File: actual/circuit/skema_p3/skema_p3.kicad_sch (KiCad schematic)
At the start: 0 parts

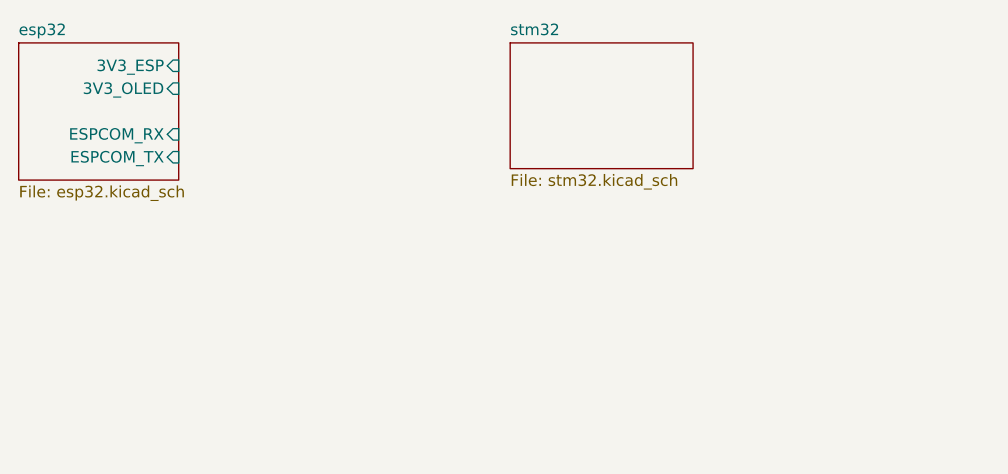
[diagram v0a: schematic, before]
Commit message: P3 in KiCAD
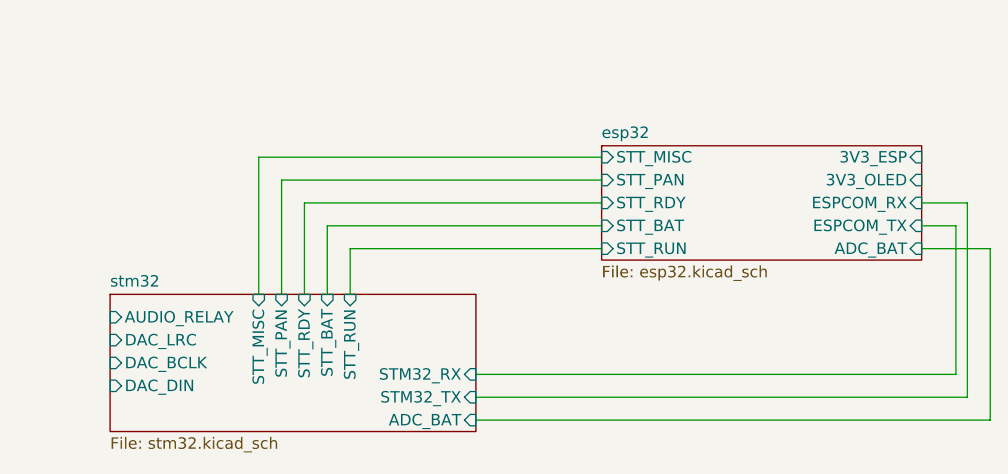
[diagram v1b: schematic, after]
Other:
- sheet esp32 ports: added ADC_BAT, STT_BAT, STT_MISC, STT_PAN, STT_RDY, STT_RUN; removed none
- sheet stm32 ports: added ADC_BAT, AUDIO_RELAY, DAC_BCLK, DAC_DIN, DAC_LRC, STM32_RX, STM32_TX, STT_BAT, STT_MISC, STT_PAN, STT_RDY, STT_RUN; removed none
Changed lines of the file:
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@@
 (kicad_sch (version 20211123) (generator eeschema)
-  (paper "User" 150.012 99.9998)
+  (paper "User" 150.012 150.012)
   (title_block
     (title "Audiometri Base Schematic")
@@
     (rev "P3 v2")
   )
-  (sheet (at 16.51 16.51) (size 17.78 15.24) (fields_autoplaced)
+  (wire (pts (xy 67.31 58.42) (xy 124.46 58.42))
+    (stroke (width 0) (type default) (color 0 0 0 0))
+  )
+  (wire (pts (xy 48.26 34.29) (xy 81.28 34.29))
+    (stroke (width 0) (type default) (color 0 0 0 0))
+  )
+  (wire (pts (xy 67.31 55.88) (xy 121.92 55.88))
+    (stroke (width 0) (type default) (color 0 0 0 0))
+  )
+  (wire (pts (xy 120.65 53.34) (xy 120.65 36.83))
+    (stroke (width 0) (type default) (color 0 0 0 0))
+  )
+  (wire (pts (xy 50.8 44.45) (xy 50.8 36.83))
+    (stroke (width 0) (type default) (color 0 0 0 0))
+  )
+  (wire (pts (xy 53.34 39.37) (xy 81.28 39.37))
+    (stroke (width 0) (type default) (color 0 0 0 0))
+  )
+  (wire (pts (xy 67.31 53.34) (xy 120.65 53.34))
+    (stroke (width 0) (type default) (color 0 0 0 0))
+  )
+  (wire (pts (xy 45.72 44.45) (xy 45.72 31.75))
+    (stroke (width 0) (type default) (color 0 0 0 0))
+  )
+  (wire (pts (xy 116.84 36.83) (xy 120.65 36.83))
+    (stroke (width 0) (type default) (color 0 0 0 0))
+  )
+  (wire (pts (xy 124.46 58.42) (xy 124.46 39.37))
+    (stroke (width 0) (type default) (color 0 0 0 0))
+  )
+  (wire (pts (xy 43.18 29.21) (xy 81.28 29.21))
+    (stroke (width 0) (type default) (color 0 0 0 0))
+  )
+  (wire (pts (xy 50.8 36.83) (xy 81.28 36.83))
+    (stroke (width 0) (type default) (color 0 0 0 0))
+  )
+  (wire (pts (xy 48.26 44.45) (xy 48.26 34.29))
+    (stroke (width 0) (type default) (color 0 0 0 0))
+  )
+  (wire (pts (xy 124.46 39.37) (xy 116.84 39.37))
+    (stroke (width 0) (type default) (color 0 0 0 0))
+  )
+  (wire (pts (xy 43.18 44.45) (xy 43.18 29.21))
+    (stroke (width 0) (type default) (color 0 0 0 0))
+  )
+  (wire (pts (xy 53.34 44.45) (xy 53.34 39.37))
+    (stroke (width 0) (type default) (color 0 0 0 0))
+  )
+  (wire (pts (xy 45.72 31.75) (xy 81.28 31.75))
+    (stroke (width 0) (type default) (color 0 0 0 0))
+  )
+  (wire (pts (xy 121.92 55.88) (xy 121.92 34.29))
+    (stroke (width 0) (type default) (color 0 0 0 0))
+  )
+  (wire (pts (xy 121.92 34.29) (xy 116.84 34.29))
+    (stroke (width 0) (type default) (color 0 0 0 0))
+  )
+  (sheet (at 81.28 27.94) (size 35.56 12.7) (fields_autoplaced)
     (stroke (width 0.1524) (type solid) (color 0 0 0 0))
     (fill (color 0 0 0 0.0000))
-    (property "Sheet name" "esp32" (id 0) (at 16.51 15.7984 0)
+    (property "Sheet name" "esp32" (id 0) (at 81.28 27.2284 0)
       (effects (font (size 1.27 1.27)) (justify left bottom))
     )
-    (property "Sheet file" "esp32.kicad_sch" (id 1) (at 16.51 32.3346 0)
+    (property "Sheet file" "esp32.kicad_sch" (id 1) (at 81.28 41.2246 0)
       (effects (font (size 1.27 1.27)) (justify left top))
     )
-    (pin "3V3_ESP" input (at 34.29 19.05 0)
-      (effects (font (size 1.27 1.27)) (justify right))
-    )
-    (pin "ESPCOM_RX" input (at 34.29 26.67 0)
-      (effects (font (size 1.27 1.27)) (justify right))
-    )
-    (pin "ESPCOM_TX" input (at 34.29 29.21 0)
-      (effects (font (size 1.27 1.27)) (justify right))
-    )
-    (pin "3V3_OLED" input (at 34.29 21.59 0)
-      (effects (font (size 1.27 1.27)) (justify right))
-    )
-  )
-  (sheet (at 71.12 16.51) (size 20.32 13.97) (fields_autoplaced)
+    (pin "3V3_ESP" input (at 116.84 29.21 0)
+      (effects (font (size 1.27 1.27)) (justify right))
+    )
+    (pin "ESPCOM_RX" input (at 116.84 34.29 0)
+      (effects (font (size 1.27 1.27)) (justify right))
+    )
+    (pin "ESPCOM_TX" input (at 116.84 36.83 0)
+      (effects (font (size 1.27 1.27)) (justify right))
+    )
+    (pin "3V3_OLED" input (at 116.84 31.75 0)
+      (effects (font (size 1.27 1.27)) (justify right))
+    )
+    (pin "STT_MISC" input (at 81.28 29.21 180)
+      (effects (font (size 1.27 1.27)) (justify left))
+    )
+    (pin "STT_PAN" input (at 81.28 31.75 180)
+      (effects (font (size 1.27 1.27)) (justify left))
+    )
+    (pin "STT_RDY" input (at 81.28 34.29 180)
+      (effects (font (size 1.27 1.27)) (justify left))
+    )
+    (pin "STT_BAT" input (at 81.28 36.83 180)
+      (effects (font (size 1.27 1.27)) (justify left))
+    )
+    (pin "STT_RUN" input (at 81.28 39.37 180)
+      (effects (font (size 1.27 1.27)) (justify left))
+    )
+    (pin "ADC_BAT" input (at 116.84 39.37 0)
+      (effects (font (size 1.27 1.27)) (justify right))
+    )
+  )
+  (sheet (at 26.67 44.45) (size 40.64 15.24) (fields_autoplaced)
     (stroke (width 0.1524) (type solid) (color 0 0 0 0))
     (fill (color 0 0 0 0.0000))
-    (property "Sheet name" "stm32" (id 0) (at 71.12 15.7984 0)
+    (property "Sheet name" "stm32" (id 0) (at 26.67 43.7384 0)
       (effects (font (size 1.27 1.27)) (justify left bottom))
     )
-    (property "Sheet file" "stm32.kicad_sch" (id 1) (at 71.12 31.0646 0)
+    (property "Sheet file" "stm32.kicad_sch" (id 1) (at 26.67 60.2746 0)
       (effects (font (size 1.27 1.27)) (justify left top))
+    )
+    (pin "STT_MISC" input (at 43.18 44.45 90)
+      (effects (font (size 1.27 1.27)) (justify right))
+    )
+    (pin "STM32_TX" input (at 67.31 55.88 0)
+      (effects (font (size 1.27 1.27)) (justify right))
+    )
+    (pin "STM32_RX" input (at 67.31 53.34 0)
+      (effects (font (size 1.27 1.27)) (justify right))
+    )
+    (pin "AUDIO_RELAY" input (at 26.67 46.99 180)
+      (effects (font (size 1.27 1.27)) (justify left))
+    )
+    (pin "DAC_LRC" input (at 26.67 49.53 180)
+      (effects (font (size 1.27 1.27)) (justify left))
+    )
+    (pin "DAC_BCLK" input (at 26.67 52.07 180)
+      (effects (font (size 1.27 1.27)) (justify left))
+    )
+    (pin "DAC_DIN" input (at 26.67 54.61 180)
+      (effects (font (size 1.27 1.27)) (justify left))
+    )
+    (pin "ADC_BAT" input (at 67.31 58.42 0)
+      (effects (font (size 1.27 1.27)) (justify right))
+    )
+    (pin "STT_RUN" input (at 53.34 44.45 90)
+      (effects (font (size 1.27 1.27)) (justify right))
+    )
+    (pin "STT_BAT" input (at 50.8 44.45 90)
+      (effects (font (size 1.27 1.27)) (justify right))
+    )
+    (pin "STT_RDY" input (at 48.26 44.45 90)
+      (effects (font (size 1.27 1.27)) (justify right))
+    )
+    (pin "STT_PAN" input (at 45.72 44.45 90)
+      (effects (font (size 1.27 1.27)) (justify right))
     )
   )
@@
       (reference "#PWR014") (unit 1) (value "GND") (footprint "")
     )
+    (path "/fceb2cae-0569-4abe-8ff3-ac4275c17dc7/67a8ea20-dd0e-44b2-a86f-66a8d9da2c19"
+      (reference "#PWR015") (unit 1) (value "GND") (footprint "")
+    )
+    (path "/fceb2cae-0569-4abe-8ff3-ac4275c17dc7/49a646a1-db2d-4b3c-ba38-d8c9fb0324b6"
+      (reference "#PWR016") (unit 1) (value "GND") (footprint "")
+    )
     (path "/597d0667-4207-4756-9f1e-dc2b80c39ef1/35709dbc-6113-4681-a2fe-9607a1e10ff5"
       (reference "Brd1") (unit 1) (value "SSD1306") (footprint "")
@@
       (reference "C10") (unit 1) (value "22pF") (footprint "")
     )
+    (path "/fceb2cae-0569-4abe-8ff3-ac4275c17dc7/3715e4a1-45ab-4740-a9d4-9a3c72d43d6e"
+      (reference "C11") (unit 1) (value "4.7uF") (footprint "")
+    )
     (path "/597d0667-4207-4756-9f1e-dc2b80c39ef1/053eb1c6-8a54-44cc-bb35-25e43aeee1de"
       (reference "J1") (unit 1) (value "Conn_01x04_Male") (footprint "")
@@
       (reference "R16") (unit 1) (value "0") (footprint "")
     )
+    (path "/fceb2cae-0569-4abe-8ff3-ac4275c17dc7/ade5cf3a-b44c-4da7-abf1-184250d94d06"
+      (reference "R17") (unit 1) (value "10K") (footprint "")
+    )
     (path "/597d0667-4207-4756-9f1e-dc2b80c39ef1/87119be6-3888-407e-976f-44367c5113e4"
       (reference "SW1") (unit 1) (value "SW_Push") (footprint "")
@@
     )
     (path "/fceb2cae-0569-4abe-8ff3-ac4275c17dc7/9f5ba256-0014-4fa0-a0e3-e794866b7f53"
-      (reference "U?") (unit 1) (value "STM32F303RBTx") (footprint "Package_QFP:LQFP-64_10x10mm_P0.5mm")
-    )
-  )
+      (reference "U3") (unit 1) (value "STM32F303RBTx") (footprint "Package_QFP:LQFP-64_10x10mm_P0.5mm")
+    )
+  )
